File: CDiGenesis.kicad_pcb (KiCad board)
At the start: 2 copper layers, 4 parts, among them J1 Genesis, J2 CDi, U1 ATtiny1616-M

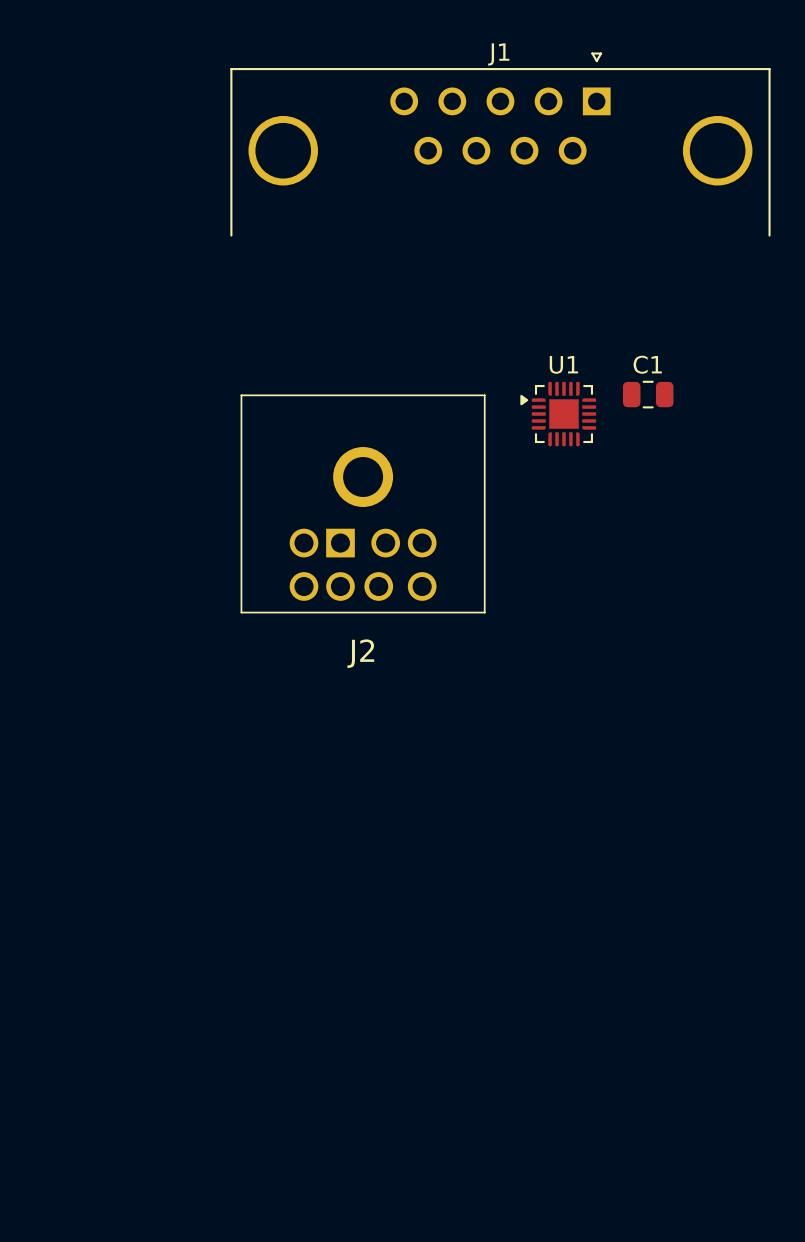
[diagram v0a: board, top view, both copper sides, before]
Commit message: Effectively finalise PCB design
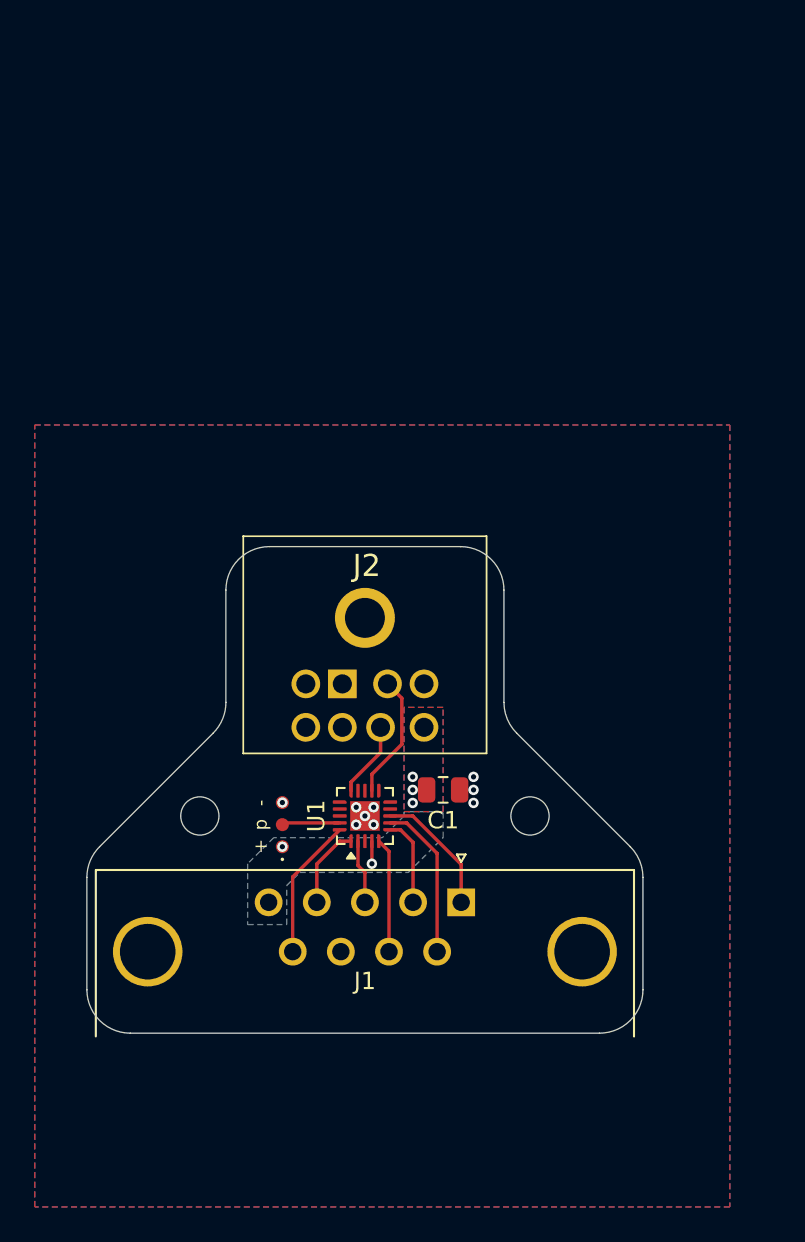
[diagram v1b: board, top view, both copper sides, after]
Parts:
- added H1: M2, MountingHole:MountingHole_2.2mm_M2, F.Cu at (144.5, 122.5)
- added H2: M2, MountingHole:MountingHole_2.2mm_M2, F.Cu at (163.5, 122.5)
- added J3: Conn_01x03, UPDI:UPDI Pads, F.Cu at (149.2, 123.0)
- moved J1 46.7 mm to (159.5, 127.5)
- moved U1 25.8 mm to (154.0, 122.5), turned to 90 degrees
- moved C1 25.6 mm to (158.5, 121.0)
- moved J2 8.11 mm to (154.0, 113.0)
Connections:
- U1 pad 1: /D_Down -> /D_Right
- U1 pad 10: /RTS -> unconnected-(U1-PB4-Pad10)
- U1 pad 15: unconnected-(U1-PC0-Pad15) -> /RTS
- U1 pad 19: unconnected-(U1-~{RESET}/PA0-Pad19) -> /UPDI
- U1 pad 20: /D_Up -> /BTN_S/C
- U1 pad 5: /D_Right -> /Select
- U1 pad 6: /BTN_A/B -> /D_Down
- U1 pad 7: /BTN_S/C -> /BTN_A/B
- U1 pad 8: /Select -> /D_Up
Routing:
- net /BTN_A/B: track 0.00 -> 9.09 mm
- net /BTN_S/C: track 0.00 -> 8.13 mm
- net /D_Up: track 0.00 -> 7.43 mm
- net /RXD: track 0.00 -> 7.21 mm
- net /Select: track 0.00 -> 6.60 mm
- net /D_Down: track 0.00 -> 5.07 mm
- net /D_Right: track 0.00 -> 4.72 mm
- net /RTS: track 0.00 -> 4.35 mm
- net /D_Left: track 0.00 -> 3.69 mm
- net /UPDI: track 0.00 -> 3.34 mm
- net +5V: track 0.00 -> 1.30 mm, vias 0 -> 5
- net GND: vias 0 -> 9
- added copper zone on B.Cu, net +5V
- added copper zone on F.Cu, net +5V
- added copper zone on B.Cu, net GND
- added copper zone on F.Cu, net GND
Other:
- board outline added: 32 x 28 mm
- board text added: "+"
- board text added: "-"
- board text added: "p"
